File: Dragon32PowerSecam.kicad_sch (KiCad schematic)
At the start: 6 parts

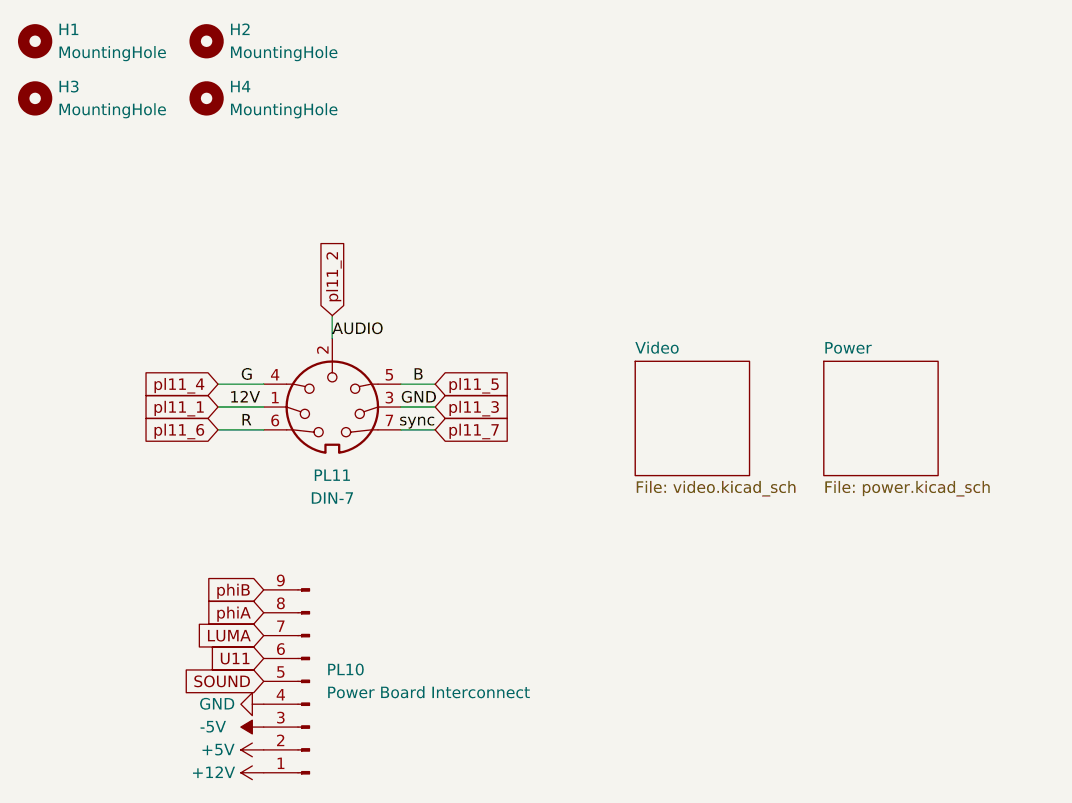
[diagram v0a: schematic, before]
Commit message: update labelling
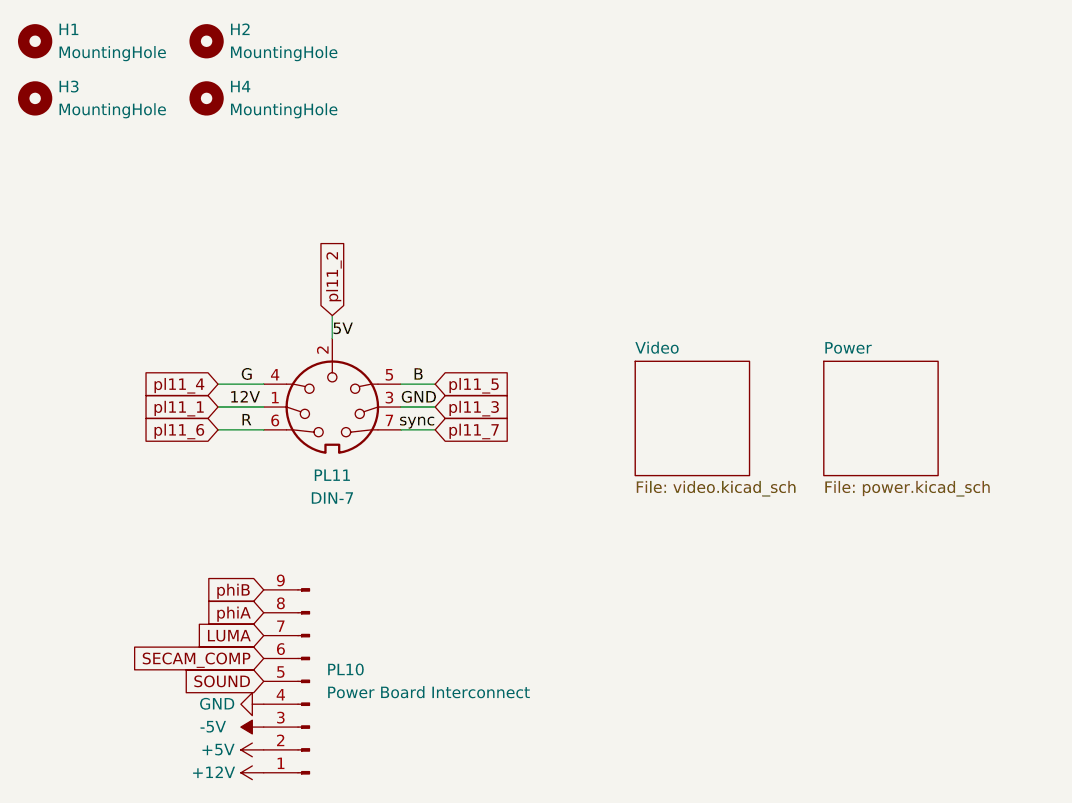
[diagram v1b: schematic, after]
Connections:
- net U11 renamed SECAM_COMP
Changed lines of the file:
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@@
 		)
 	)
-	(label "AUDIO"
+	(label "5V"
 		(at 55.88 54.61 0)
 		(effects
@@
 		)
 	)
-	(global_label "U11"
+	(global_label "SECAM_COMP"
 		(shape input)
 		(at 48.26 90.17 180)
@@
 		)
 		(property "Intersheetrefs" "${INTERSHEET_REFS}"
-			(at 41.5253 90.17 0)
-			(effects
-				(font
+			(at 32.8168 90.17 0)
+			(effects
+				(font
